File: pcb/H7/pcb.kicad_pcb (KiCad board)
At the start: 4 copper layers, 43 x 40.1 mm, 83 parts, among them u1 ESP8285, u2 STMH723VGT6, u3 LDL1117S33R, u4 TPS5430DDAR, u5 DPS368XTSA1, u6 LIS3MDLTR, u7 ICM-42688-P, u8 W25Q128FVSIG

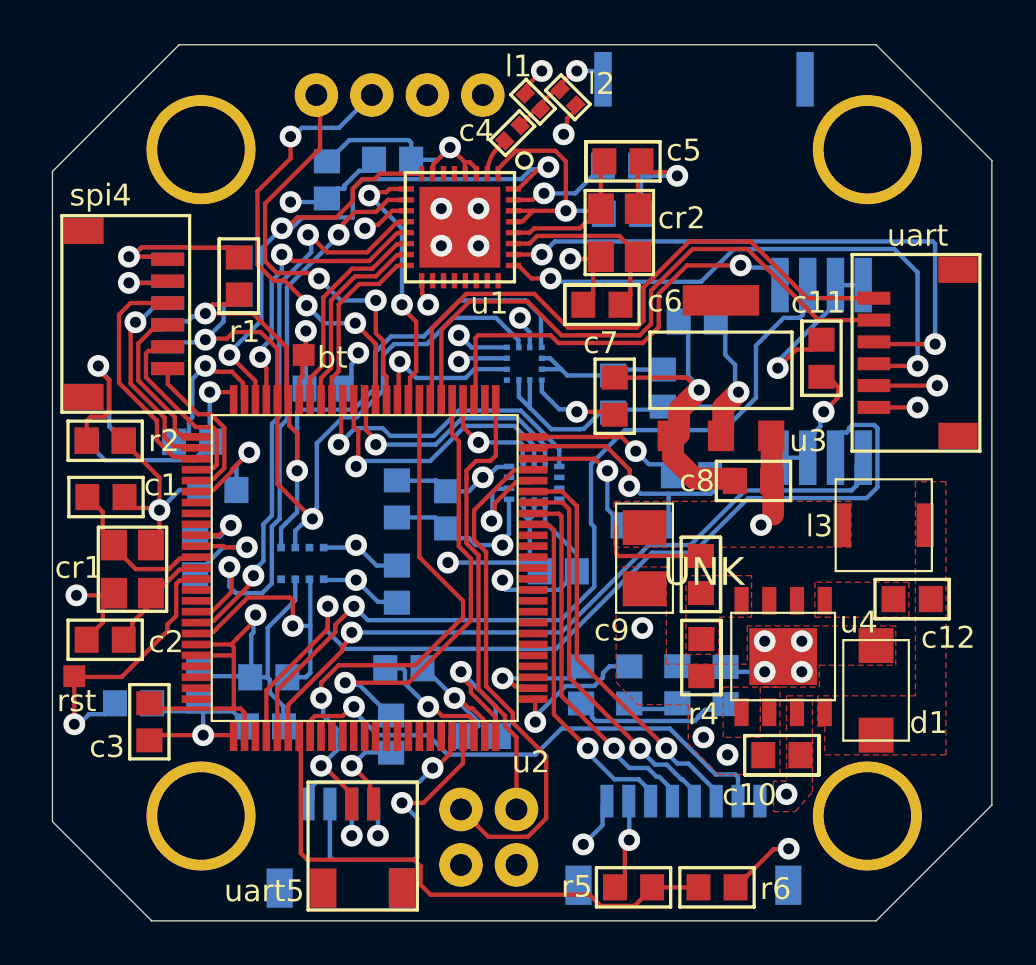
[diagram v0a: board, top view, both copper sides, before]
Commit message: pcb updated
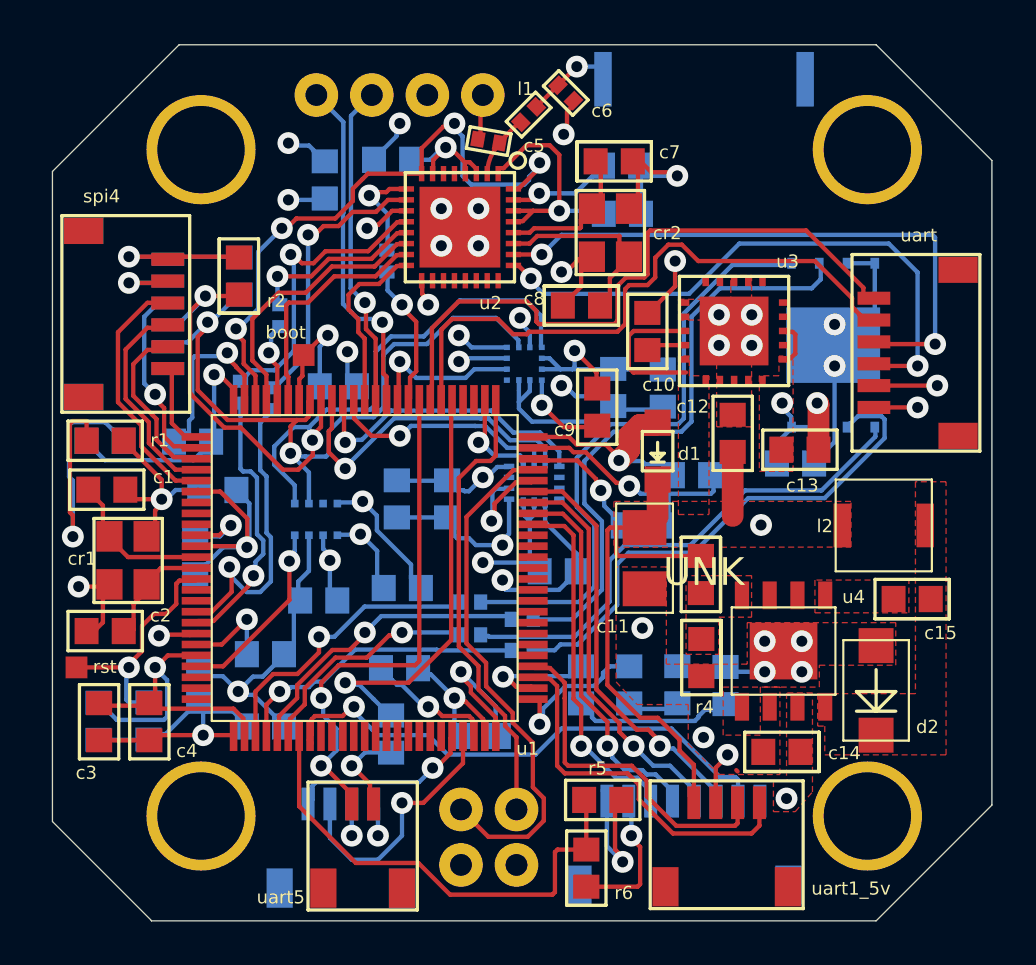
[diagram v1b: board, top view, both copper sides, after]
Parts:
- removed l3: 10 uH, PcbLib1:inductor
- removed pwr: green LED, PcbLib1:0603
- added c34: 0.1 uF, PcbLib1:0603, B.Cu at (133.4, 108.2)
- added c35: 1 uF, PcbLib1:0603, B.Cu at (133.6, 114.1)
- added c36: 0.1 uF, PcbLib1:0603, B.Cu at (131.3, 115.8)
- added c37: 0.1 uF, PcbLib1:0603, B.Cu at (129.0, 115.8)
- added d2: SS34, PcbLib1:SS34, F.Cu at (165.8, 114.4)
- added pwr1: green LED, PcbLib1:0603, B.Cu at (129.5, 102.9)
- added r13: 33 Ohm, PcbLib1:0402, B.Cu at (146.1, 112.0)
- added r14: 33 Ohm, PcbLib1:0402, B.Cu at (142.3, 94.9)
- added r15: 10 kOhm, PcbLib1:0603, B.Cu at (140.2, 100.5)
- added r16: 100 Ohm, PcbLib1:0603, B.Cu at (142.4, 116.4)
- added r17: 33 Ohm, PcbLib1:0402, B.Cu at (137.4, 97.4)
- added r18: 33 Ohm, PcbLib1:0402, B.Cu at (137.1, 101.2)
- added r19: 47 Ohm, PcbLib1:0603, B.Cu at (136.9, 112.7)
- added r20: 3 kOhm, PcbLib1:0603, B.Cu at (135.7, 95.7)
- added r21: 33 Ohm, PcbLib1:0402, B.Cu at (135.6, 100.9)
- added uart1_5v: JST SH-4, PcbLib1:sh1.0-4, F.Cu at (158.0, 121.0)
- c10, c20: value 10 uF -> 1 uF
- c11: value 0.1 uF -> 100 uF; footprint PcbLib1:0603 -> PcbLib1:1206
- c12: value 0.01 uF -> 10 uF
- c13: value 0.1 uF -> 47 uF; moved to F.Cu
- c14: value 0.1 uF -> 10 uF; moved to F.Cu
- c15: value 0.1 uF -> 0.01 uF; moved to F.Cu
- c16: value 1 uF -> 0.1 uF
- c18, c3: value 0.1 uF -> 1 uF
- c21: value 0.1 uF -> 2.2 uF
- c22: value 0.1 uF -> 0.01 uF
- c23, c25, c32: value 2.2 uF -> 0.1 uF
- c27: value 1 uF -> 2.2 uF
- c28: value 4.7 uF -> 2.2 uF
- c29: value 1 uF -> 10 uF
- c33: value 0.01 uF -> 0.1 uF
- c4: value 5.6 pF, tdb -> 0.1 uF; footprint PcbLib1:0402 -> PcbLib1:0603
- c5, c6: value 18 pF -> tbd; footprint PcbLib1:0603 -> PcbLib1:0402
- c7: value 0.1 uF -> 18 pF
- c8: value 1 uF -> 18 pF
- c9: value 100 uF -> 0.1 uF; footprint PcbLib1:1206 -> PcbLib1:0603
- d1: value SS34 -> Comment; footprint PcbLib1:SS34 -> PcbLib1:SOD-323
- l1: value tbd -> tdb
- l2: value tbd -> 10 uH; footprint PcbLib1:0402 -> PcbLib1:inductor
- led1: value orange LED -> blue LED
- led2: value blue LED -> orange LED
- r1, r7: value 3 kOhm -> 1 kOhm
- r10: value 12 kOhm -> 33 Ohm; footprint PcbLib1:0603 -> PcbLib1:0402
- r11, r12: value 1 kOhm -> 33 Ohm; footprint PcbLib1:0603 -> PcbLib1:0402
- r2: value 1 kOhm -> 3 kOhm
- r5: value 3 kOhm -> 680 Ohm
- r6: value 6.8 kOhm -> 5.1 kOhm
- r8: value 10 kOhm -> 1 kOhm
- r9: value 100 Ohm -> 12 kOhm
- u1: value ESP8285 -> STMH723VGT6; footprint PcbLib1:esp8285 -> PcbLib1:lqfp100
- u2: value STMH723VGT6 -> ESP8285; footprint PcbLib1:lqfp100 -> PcbLib1:esp8285
- u3: value LDL1117S33R -> TPS7A4700; footprint PcbLib1:ams1117 -> PcbLib1:TPS7A470
- u5: value DPS368XTSA1 -> Comment; footprint PcbLib1:DPS368 -> PcbLib1:W25N
- u6: value LIS3MDLTR -> ICM-42688-P; footprint PcbLib1:lis3mdl -> PcbLib1:icm42688
- u7: value ICM-42688-P -> LIS3MDLTR; footprint PcbLib1:icm42688 -> PcbLib1:lis3mdl
- u8: value W25Q128FVSIG -> DPS368XTSA1; footprint PcbLib1:w25q -> PcbLib1:DPS368
- moved c15 33.1 mm to (166.5, 110.5), turned to -90 degrees
- moved c4 31.8 mm to (131.3, 116.1), turned to 180 degrees
- moved r7 29.1 mm to (157.9, 114.4)
- moved c16 29.0 mm to (160.9, 104.3), turned to -90 degrees
- moved c14 28.7 mm to (160.5, 117.5)
- moved r9 28.2 mm to (153.2, 90.3), turned to 90 degrees
- moved c17 27.9 mm to (156.4, 104.5), turned to 90 degrees
- moved u1 27.8 mm to (132.3, 117.5)
- moved u2 27.8 mm to (147.0, 93.9)
- moved c13 27.8 mm to (161.1, 103.4), turned to 90 degrees
- moved c18 26.7 mm to (153.2, 92.6)
- moved u5 26.6 mm to (162.7, 98.7)
- moved u8 24.5 mm to (138.7, 106.7), turned to 90 degrees
- moved l2 24.4 mm to (165.0, 107.1), turned to -90 degrees
- moved c19 24.0 mm to (154.8, 100.6), turned to 180 degrees
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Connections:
- c12 pad 1: dcdc_boot -> gnd
- c15 pad 1: gnd -> dcdc_boot
- c17 pad 1: nrst -> gnd
- c20 pad 1: gnd -> vcc
- c24 pad 1: vcc -> gnd
- c25 pad 1: gnd -> vcc
- c28 pad 1: gnd -> vcc
- c29 pad 1: vcc -> gnd
- c33 pad 1: vcc -> gnd
- c4 pad 1: antcap -> vcc
- c5 pad 1: gnd -> antcap
- c6 pad 1: xtal_out -> gnd
- c8 pad 1: gnd -> xtal_out
- l1 pad 1: gnd -> antcap
- led1 pad 1: led2r -> led1r
- led2 pad 1: led1r -> led2r
- r1 pad 1: vcc -> gnd
- r10 pad 1: gnd -> miso1_2
- r11 pad 1: led1r -> sck1_2
- r12 pad 1: led2r -> nss1_2
- r2 pad 1: gnd -> vcc
- r7 pad 1: sda -> led2r
- r8 pad 1: gnd -> led1r
- r9 pad 1: tx5_1 -> gnd
- spi4 pad 1: mosi4 -> sck4
- u8 pad 1: cs2 -> gnd
- uart pad 1: rx4 -> tx4
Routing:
- net sck6: track 43.5 -> 0.00 mm, vias 1 -> 0
- net miso6: track 40.6 -> 0.00 mm, vias 1 -> 0
- net mosi6: track 33.2 -> 0.00 mm, vias 1 -> 0
- net nss1_2: track 0.00 -> 28.1 mm
- net miso1_2: track 0.00 -> 27.8 mm
- net miso2: track 26.8 -> 0.00 mm, vias 2 -> 0
- net v5: track 39.3 -> 65.3 mm
- net mosi2: track 25.8 -> 0.00 mm, vias 2 -> 0
- net sck1_2: track 0.00 -> 24.1 mm
- net mosi1_2: track 0.00 -> 23.5 mm
- net cs2: track 20.2 -> 0.00 mm, vias 1 -> 0
- net tx1: track 0.00 -> 17.1 mm
- net rx1: track 0.00 -> 15.9 mm
- net mosi3: track 0.00 -> 14.9 mm, vias 0 -> 1
- net miso: track 14.8 -> 0.00 mm, vias 1 -> 0
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- added copper zone on F.Cu, net vcc
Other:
- board text added: "boot"
- board text removed: "bt"

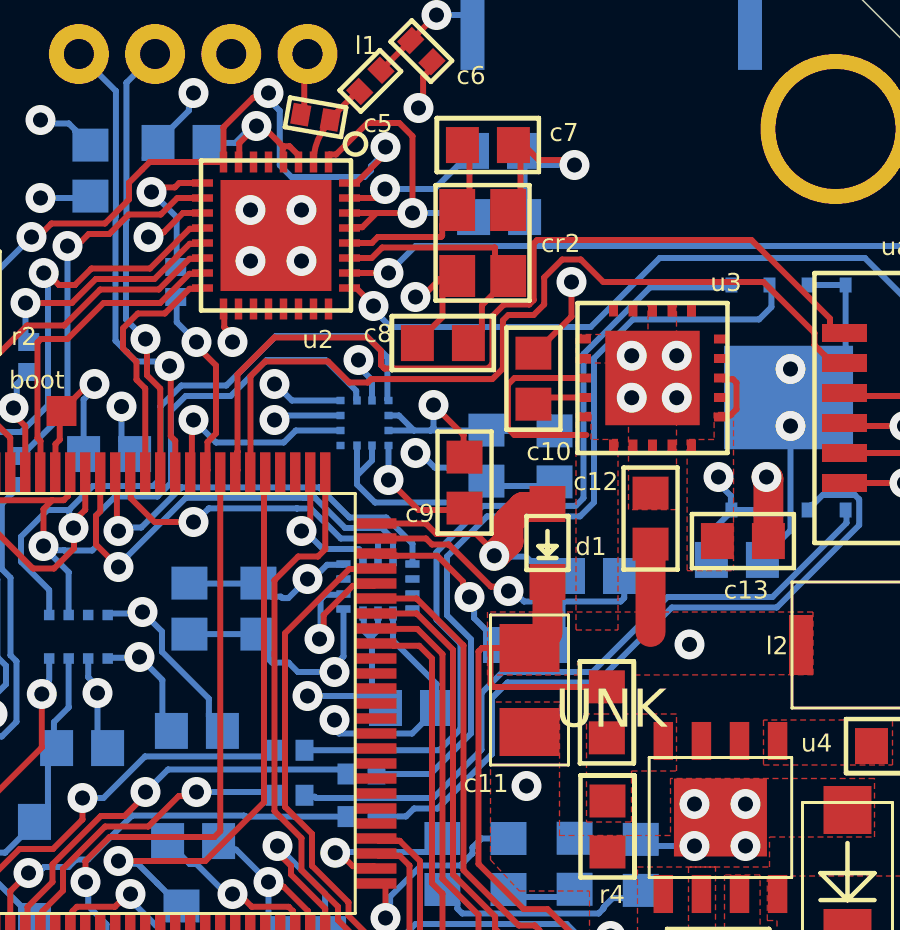
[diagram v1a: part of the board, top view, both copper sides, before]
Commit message: schematic updated
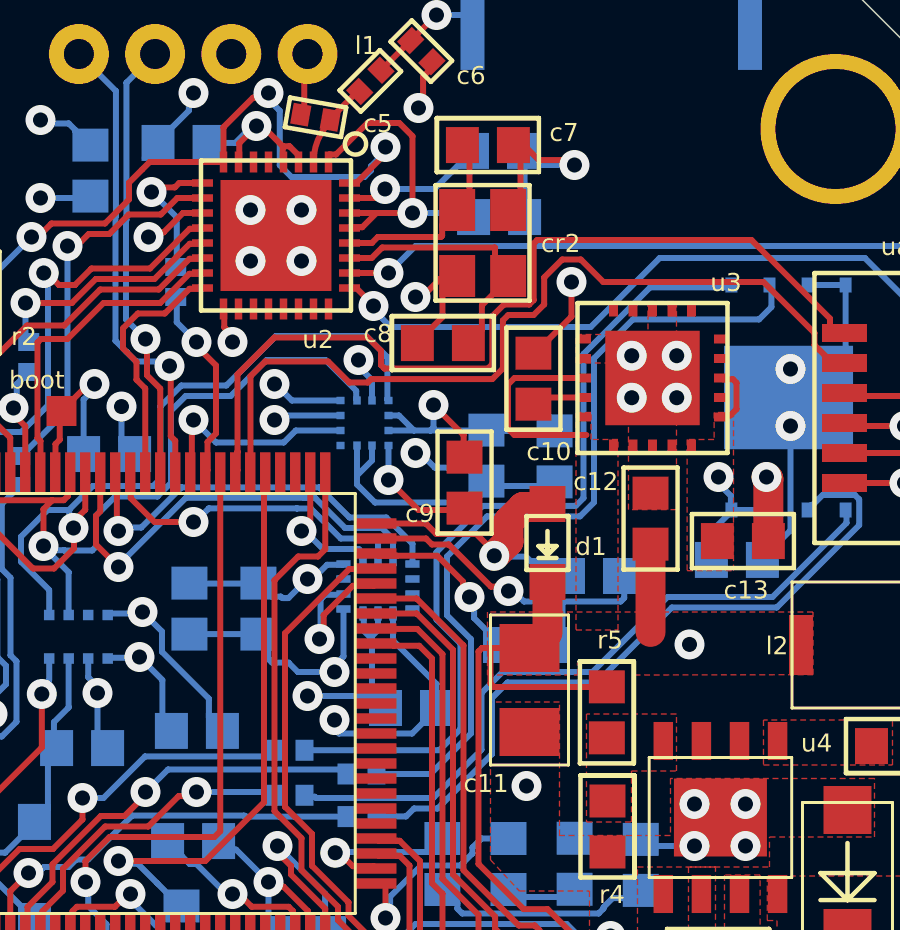
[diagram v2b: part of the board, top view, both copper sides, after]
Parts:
- renumbered UNK to r5
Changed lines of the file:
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@@
 		)
 		(property "Value" "tbd"
-			(at 1.301473 5.27861 0)
+			(at 1.301473 5.278609 0)
 			(unlocked yes)
 			(layer "F.SilkS")
@@
 		(layer "F.Cu")
 		(at 156.8159 109.08582)
-		(property "Reference" "UNK"
-			(at 0 0 0)
+		(property "Reference" "r5"
+			(at -0.0298 -2.29222 0)
 			(layer "F.SilkS")
 			(effects
 				(font
-					(size 1.27 1.27)
+					(size 0.6 0.6)
 					(thickness 0.15)
 				)
@@
 	)
 	(gr_rect
-		(start 143.8011 95.1536)
-		(end 147.5011 91.4536)
+		(start 143.8011 91.4536)
+		(end 147.5011 95.1536)
 		(stroke
 			(width 0)
